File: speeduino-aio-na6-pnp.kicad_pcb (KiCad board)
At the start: 4 copper layers, 154 x 160 mm, 194 parts, among them J1 CONN_BLACK, J2 CONN_GREY, J3 SWD, P1 USB_C_Plug_USB2.0, Q1 AO3401A, Q2 Q_PNP_BEC, U1 VNLD5090, U10 USBLC6-2SC6, U11 MCP2551-I-SN, U12 STM32F429ZGTx, U13 VNLD5090, U14 VNLD5090, U15 MC33814, U2 VNLD5090, U3 VNLD5090, U4 TC4424A, U5 TC4424A, U6 SP720, U7 MPX4250, U8 TPS5430DDA, U9 TPS5430DDA, Y1 25mhz

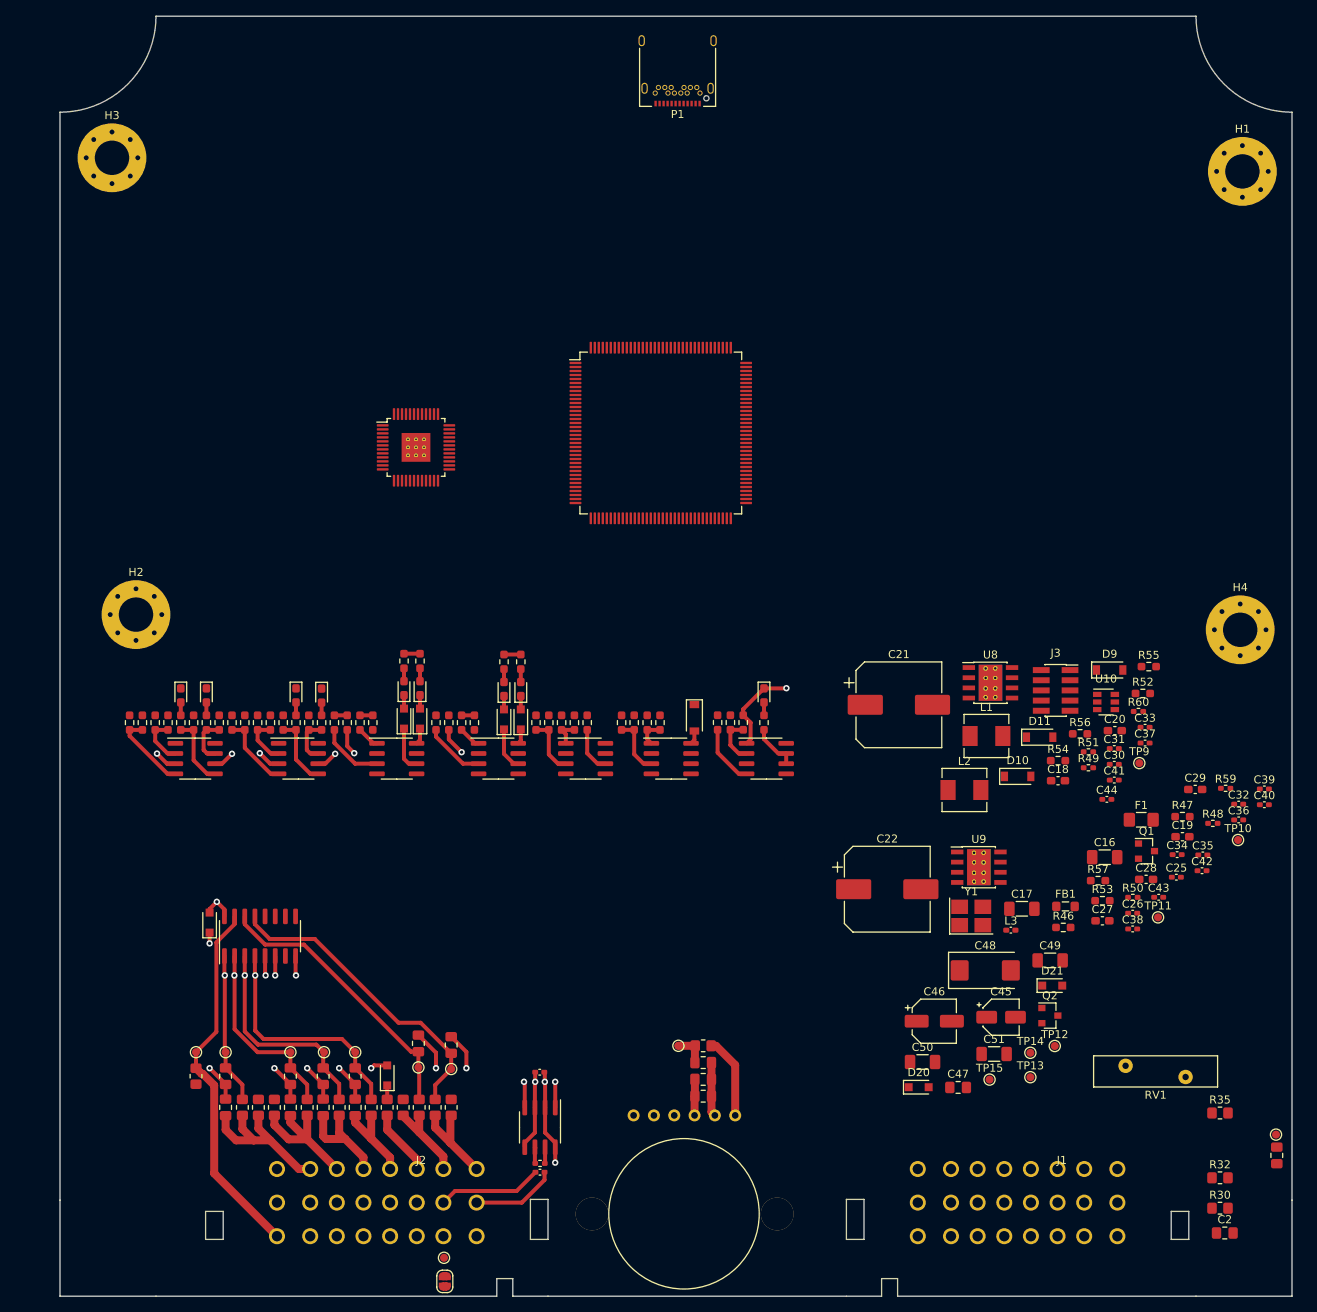
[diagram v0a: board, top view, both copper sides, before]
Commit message: Layout p much finished.. Time for some stretch goals..?
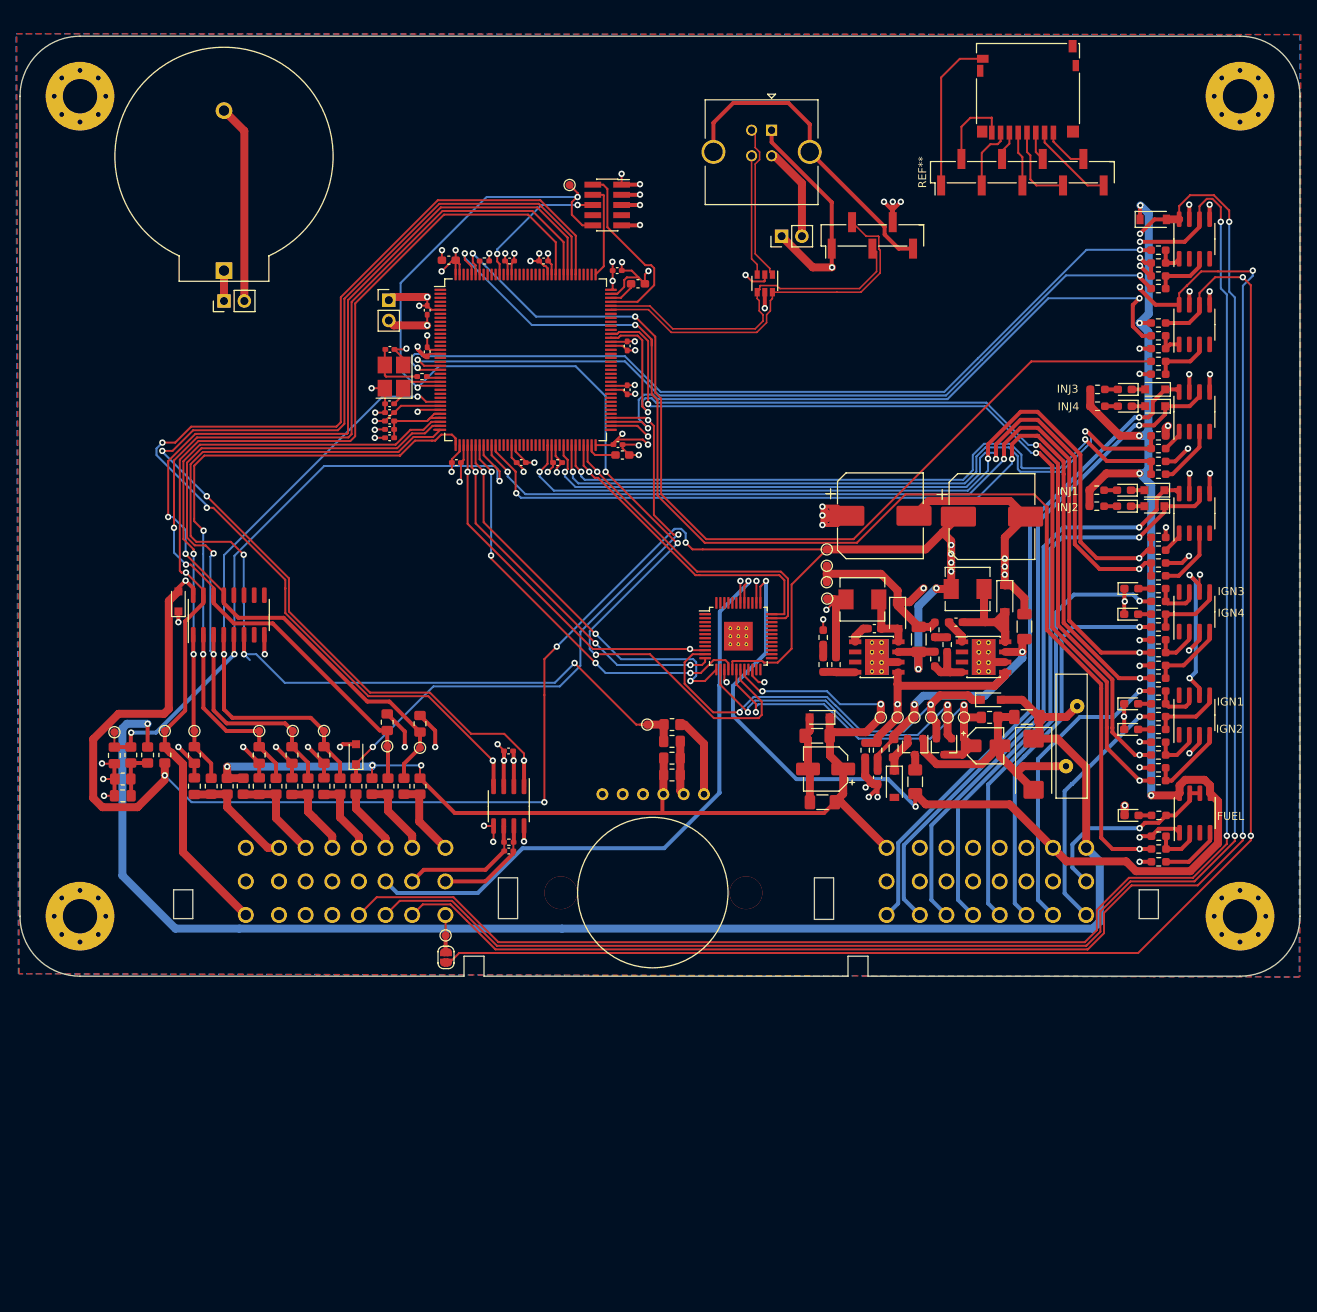
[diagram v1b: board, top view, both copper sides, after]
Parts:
- removed C42: 100n, Capacitor_SMD:C_0402_1005Metric_Pad0.74x0.62mm_HandSolder
- removed P1: USB_C_Plug_USB2.0, Connector_USB:USB_C_Receptacle_Amphenol_12401548E4-2A
- removed R48, R51: 5.1k, Resistor_SMD:R_0402_1005Metric_Pad0.72x0.64mm_HandSolder
- removed R49, R50: 22, Resistor_SMD:R_0402_1005Metric_Pad0.72x0.64mm_HandSolder
- added J4: USB_B, Connector_USB:USB_B_Amphenol_MUSB-D511_Vertical_Rugged, F.Cu at (109.0, 34.2)
- added J5: USB_EXT, Connector_PinHeader_2.54mm:PinHeader_1x05_P2.54mm_Vertical_SMD_Pin1Left, F.Cu at (121.5, 47.4)
- added REF**: PinHeader_1x09_P2.54mm_Vertical_SMD_Pin1Left, Connector_PinHeader_2.54mm:PinHeader_1x09_P2.54mm_Vertical_SMD_Pin1Left, F.Cu at (140.3, 39.5)
- added REF**: PinHeader_1x02_P2.54mm_Vertical, Connector_PinHeader_2.54mm:PinHeader_1x02_P2.54mm_Vertical, F.Cu at (110.2, 47.5)
- added REF**: PinHeader_1x02_P2.54mm_Vertical, Connector_PinHeader_2.54mm:PinHeader_1x02_P2.54mm_Vertical, F.Cu at (61.1, 55.5)
- added REF**: PinHeader_1x02_P2.54mm_Vertical, Connector_PinHeader_2.54mm:PinHeader_1x02_P2.54mm_Vertical, F.Cu at (40.5, 55.6)
- added REF**: microSD_HC_Hirose_DM3D-SF, Connector_Card:microSD_HC_Hirose_DM3D-SF, F.Cu at (141.0, 29.2)
- added REF**: BatteryHolder_ComfortableElectronic_CH273-2450_1x2450, Battery:BatteryHolder_ComfortableElectronic_CH273-2450_1x2450, F.Cu at (40.5, 51.8)
- added TP18: TP_BUCK_EN, TestPoint:TestPoint_Pad_D1.0mm, F.Cu at (124.7, 107.7)
- added TP19: TP_PWR_GND2, TestPoint:TestPoint_Pad_D1.0mm, F.Cu at (115.8, 90.8)
- added TP20: TP_PWR_GND1, TestPoint:TestPoint_Pad_D1.0mm, F.Cu at (115.8, 88.7)
- added TP21: TP_BUCK_IN, TestPoint:TestPoint_Pad_D1.0mm, F.Cu at (126.8, 107.7)
- TP10: value TestPoint_Small -> TP_5V
- TP11: value TestPoint_Small -> TP_3V
- moved TP3 153.7 mm to (26.8, 109.5)
- moved C4 153.7 mm to (26.8, 112.4)
- moved C2 148.2 mm to (27.9, 117.5), turned to 180 degrees
- moved R30 147.3 mm to (27.9, 115.3), turned to 180 degrees
- moved R32 144.1 mm to (30.9, 112.3), turned to 270 degrees
- moved R35 143.3 mm to (28.9, 112.3), turned to 270 degrees
- moved R17 128.8 mm to (157.3, 115.5), turned to 180 degrees
- moved R21 127.1 mm to (157.3, 114.0), turned to 0 degrees
- moved R16 125.5 mm to (157.3, 112.3), turned to 180 degrees
- moved U5 125.0 mm to (161.8, 107.3), turned to 90 degrees
- moved R20 123.8 mm to (157.3, 110.8), turned to 180 degrees
- moved R29 122.2 mm to (157.3, 109.2), turned to 0 degrees
- moved R25 120.6 mm to (157.3, 107.5), turned to 180 degrees
- moved C39 119.0 mm to (61.2, 69.5), turned to 180 degrees
- moved R28 119.0 mm to (157.3, 106.0), turned to 180 degrees
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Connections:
- C20 pad 2: Net-(C20-Pad2) -> GND
- C46 pad 2: GND -> Net-(C46-Pad2)
- C50 pad 2: GND -> Net-(C46-Pad2)
- C51 pad 2: GND -> Net-(C46-Pad2)
- D20 pad 2: GND -> Net-(C46-Pad2)
- J1 pad B1: GND -> ST_SIG
- J1 pad B8: ST_SIG -> GND
- J1 pad C1: INJ-1 -> IGN-2
- J1 pad C2: INJ-2 -> IGN-1
- J1 pad C3: INJ-3 -> IGN-4
- J1 pad C4: INJ-4 -> IGN-3
- J1 pad C5: IGN-1 -> INJ-2
- J1 pad C6: IGN-2 -> INJ-1
- J1 pad C7: IGN-3 -> INJ-4
- J1 pad C8: IGN-4 -> INJ-3
- J2 pad A8: FP -> Net-(J2-PadA8)
- J2 pad B3: GND -> FP
- J2 pad C1: FAN -> TACH
- J2 pad C2: TACH -> FAN
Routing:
- net GND: track 76.9 -> 328.4 mm, vias 16 -> 80
- net +5V: track 9.22 -> 250.9 mm, vias 3 -> 14
- net BOOST: track 0.00 -> 212.5 mm, vias 0 -> 3
- net IDLE: track 1.72 -> 210.1 mm, vias 0 -> 3
- net 12v-SW: track 4.10 -> 211.1 mm, vias 0 -> 7
- net FAN: track 0.00 -> 203.4 mm, vias 0 -> 3
- net VBAT: track 0.00 -> 195.7 mm, vias 0 -> 1
- net Net-(JP1-Pad1): track 5.74 -> 191.4 mm, vias 0 -> 2
- net /FuelPump/MCU-FP: track 0.00 -> 157.0 mm, vias 0 -> 3
- net NRST: track 0.00 -> 149.3 mm, vias 0 -> 5
- net MCU-CAN-TX: track 3.23 -> 147.5 mm, vias 1 -> 3
- net MCU-CAN-RX: track 3.26 -> 146.0 mm, vias 1 -> 3
- net VPROT: track 4.52 -> 141.1 mm, vias 0 -> 5
- net /FAN+TACH/MCU-TACH: track 0.00 -> 122.7 mm, vias 0 -> 2
- net ADC-CLAMP-6: track 6.64 -> 127.5 mm, vias 1 -> 3
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- added copper zone on In2.Cu, net +3V3
- added copper zone on In2.Cu, net +5V
- added copper zone on In2.Cu, net 12v-SW
- added copper zone on B.Cu, net GND
- added copper zone on F.Cu, net GND
- added copper zone on In1.Cu, net GND
- added copper zone on In2.Cu, net USB_CONN_VBUS
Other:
- board size 154 x 160 mm -> 160 x 117.5 mm
- board text added: "FUEL"
- board text added: "IGN1"
- board text added: "IGN2"
- board text added: "IGN3"
- board text added: "IGN4"
- board text added: "INJ1"
- board text added: "INJ2"
- board text added: "INJ3"
- board text added: "INJ4"
